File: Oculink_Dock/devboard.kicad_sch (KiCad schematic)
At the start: 27 parts, among them J6 Conn_01x03, J7 Conn_01x10, J8 Conn_01x10, SW4 SW_Push, U5 W25Q128JVS, U6 RP2040, Y1 12 MHz

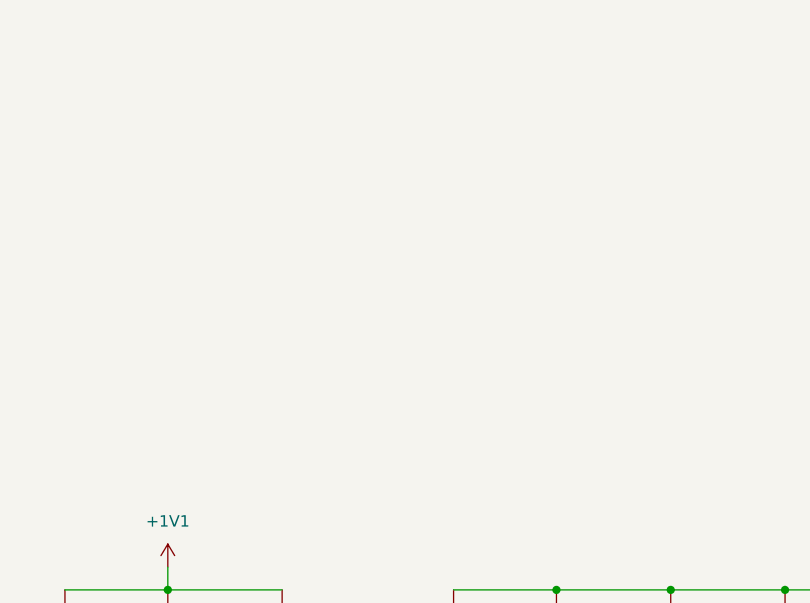
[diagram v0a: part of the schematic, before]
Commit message: Update
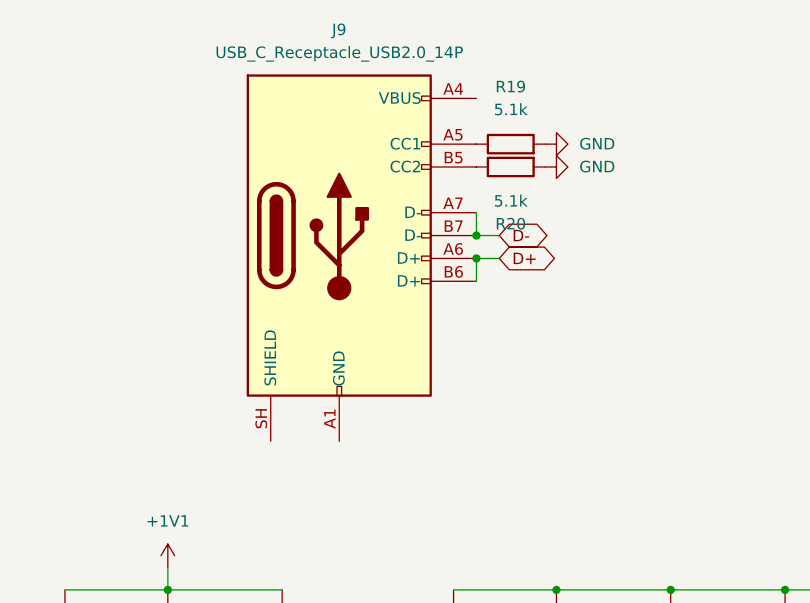
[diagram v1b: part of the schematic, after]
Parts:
- added J9: USB_C_Receptacle_USB2.0_14P, Package_DFN_QFN:WDFN-10-1EP_3x3mm_P0.5mm_EP1.8x2.5mm, symbol Connector:USB_C_Receptacle_USB2.0_14P
- added R19, R20: 5.1k, symbol Device:R
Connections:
- net D+: now also J9.A6 (D+), J9.B6 (D+)
- net D-: now also J9.A7 (D-), J9.B7 (D-)
- net GND: now also R19.2, R20.2
- new net: J9.A5 (CC1), R19.1
- new net: J9.B5 (CC2), R20.1
- new net: J9.A1 (GND), J9.A12 (GND), J9.B1 (GND), J9.B12 (GND)
- new net: J9.A4 (VBUS), J9.A9 (VBUS), J9.B4 (VBUS), J9.B9 (VBUS)
